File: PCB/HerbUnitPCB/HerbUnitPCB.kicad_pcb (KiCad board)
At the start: 2 copper layers, 43 parts, among them J1 USB_C_Receptacle_USB2.0_16P, J2 Barrel_Jack_Switch_Pin3Ring, J3 Conn_01x03_Pin, J4 SD_Card_Device, J5 Screw_Terminal_01x02, J6 Conn_01x03_Pin, SW1 SW_Push, SW2 SW_Push, SW3 SW_Push, U1 USBLC6-2P6, U2 ESP32-S3-WROOM-1, U3 AMS1117-5.0, U5 DHT11, U6 AP2112K-3.3

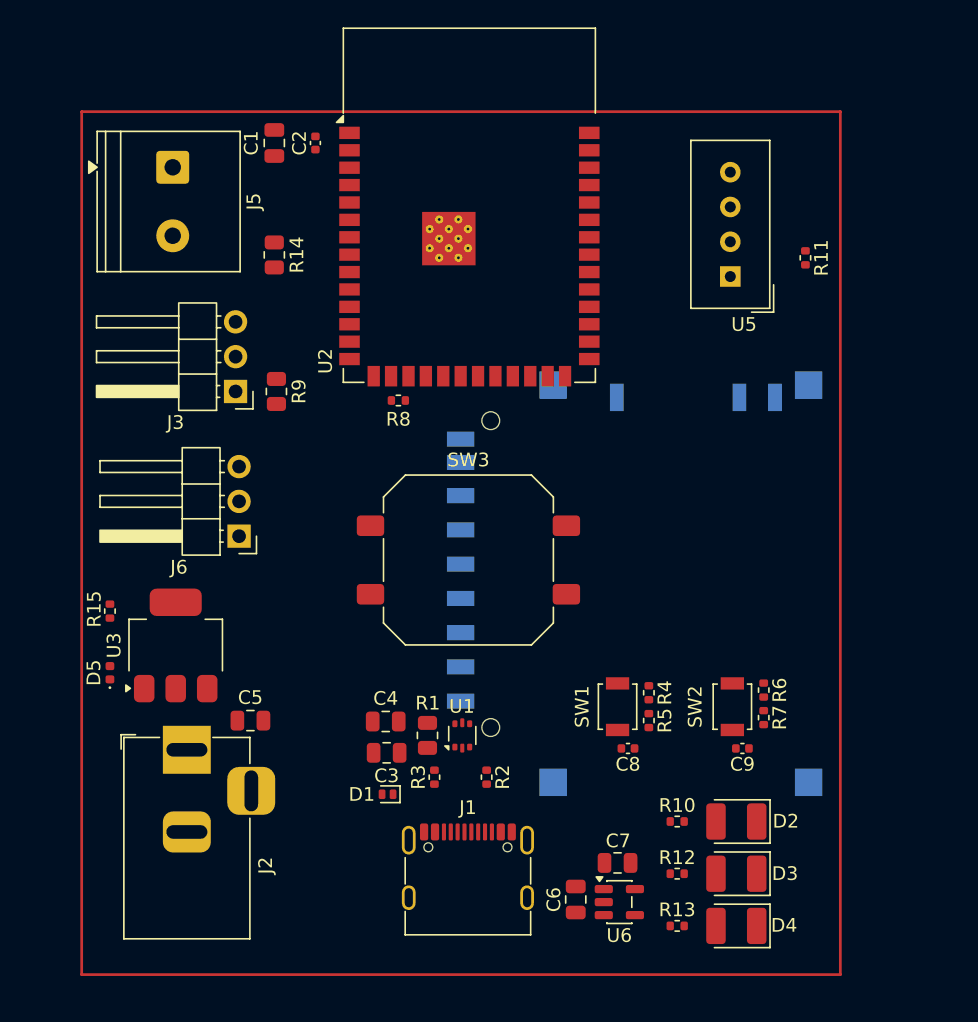
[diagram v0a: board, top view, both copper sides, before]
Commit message: PCB Routed + Silkscreen
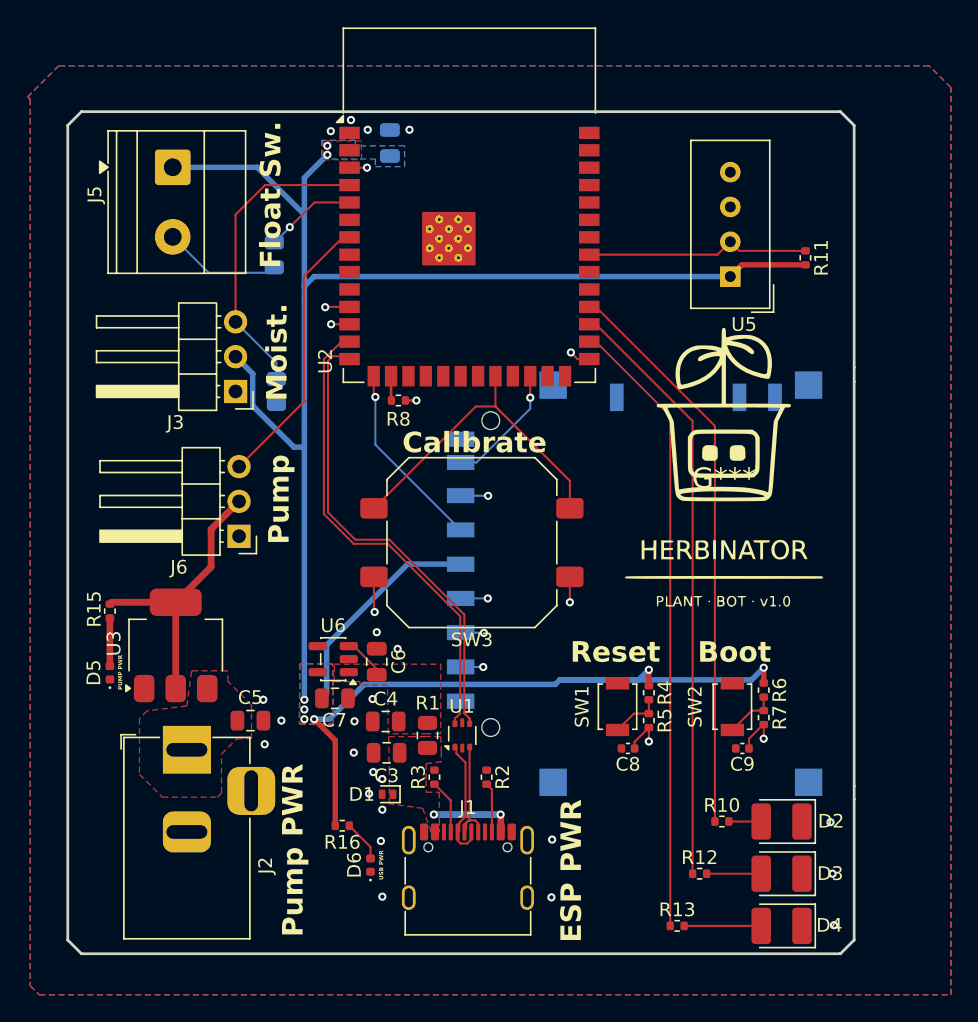
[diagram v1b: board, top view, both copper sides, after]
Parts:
- added D6: Green LED, LED_SMD:LED_0402_1005Metric, F.Cu at (160.0, 89.5)
- added G***: LOGO, LOGO, F.Cu at (185.8, 61.3)
- added G***: LOGO, LOGO, B.Cu at (167.2, 44.6)
- added G***: LOGO, LOGO, B.Cu at (184.0, 89.6)
- added R16: 2k, Resistor_SMD:R_0402_1005Metric, F.Cu at (158.0, 86.7)
- C1, C2, R14, R9: moved to B.Cu
- J5: footprint TerminalBlock_Philmore:TerminalBlock_Philmore_TB132_1x02_P5.00mm_Horizontal -> TerminalBlock_Phoenix:TerminalBlock_Phoenix_MKDS-1,5-2-5.08_1x02_P5.08mm_Horizontal
- moved U6 27.4 mm to (157.3, 74.5), turned to 180 degrees
- moved C7 23.9 mm to (157.4, 77.4), turned to 0 degrees
- moved C6 22.6 mm to (160.5, 74.7), turned to 90 degrees
- moved C1 8.44 mm to (161.4, 36.8)
- moved D2 3.30 mm to (190.0, 86.4)
- moved D3 3.30 mm to (190.0, 90.2)
- moved D4 3.30 mm to (190.0, 94.0)
- moved R10 3.26 mm to (185.7, 86.4)
- moved C2 2.55 mm to (158.5, 36.7)
- moved R12 1.64 mm to (184.0, 90.2)
- moved SW3 1.30 mm to (167.4, 66.0)
- turned C4 to 180 degrees
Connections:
- net Net-(D1-K) renamed VBUS
- net Net-(U3-VI) renamed JACK_BUS
- R10 pad 1: RedLED -> GreenLED
- R13 pad 1: GreenLED -> RedLED
- U2 pad 18: WaterRead -> unconnected-(U2-IO10-Pad18)
- U2 pad 19: RedLED -> unconnected-(U2-IO11-Pad19)
- U2 pad 20: BlueLED -> unconnected-(U2-IO12-Pad20)
- U2 pad 21: GreenLED -> unconnected-(U2-IO13-Pad21)
- U2 pad 22: unconnected-(U2-IO14-Pad22) -> CalibrationButton
- U2 pad 28: unconnected-(U2-IO35-Pad28) -> RedLED
- U2 pad 29: unconnected-(U2-IO36-Pad29) -> BlueLED
- U2 pad 30: unconnected-(U2-IO37-Pad30) -> GreenLED
- U2 pad 33: unconnected-(U2-IO40-Pad33) -> TempSensor
- U2 pad 5: TempSensor -> WaterRead
- U2 pad 6: CalibrationButton -> unconnected-(U2-IO6-Pad6)
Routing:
- net +3.3V_USB: track 0.00 -> 165.5 mm, vias 0 -> 8
- net En: track 0.00 -> 54.7 mm, vias 0 -> 2
- net RedLED: track 0.00 -> 45.4 mm
- net BlueLED: track 0.00 -> 43.5 mm
- net GreenLED: track 0.00 -> 41.6 mm
- net BootMode1: track 0.00 -> 38.8 mm, vias 0 -> 2
- net SD_CS: track 0.00 -> 34.9 mm, vias 0 -> 2
- net USB_D-: track 0.00 -> 34.7 mm
- net USB_D+: track 0.00 -> 34.0 mm
- net SD_MOSI: track 0.00 -> 30.2 mm, vias 0 -> 2
- net CalibrationButton: track 0.00 -> 23.8 mm
- net MoistureRead: track 0.00 -> 22.4 mm
- net +5V_JACK: track 0.00 -> 20.4 mm
- net PumpMotor: track 0.00 -> 20.4 mm
- net TempSensor: track 0.00 -> 16.4 mm
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- added copper zone on B.Cu, net +3.3V_USB
- added copper zone on F.Cu, net +3.3V_USB
- added copper zone on F.Cu, net +5V
- added copper zone on B.Cu, net GND
- added copper zone on F.Cu, net GND
- added copper zone on In1.Cu, net GND
- added copper zone on In2.Cu, net GND
- added copper zone on F.Cu, net JACK_BUS
- added copper zone on F.Cu, net VBUS
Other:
- board outline added: 57.4 x 61.5 mm
- copper layers 2 -> 4
- board text added: "Boot"
- board text added: "Calibrate"
- board text added: "ESP PWR"
- board text added: "Float Sw."
- board text added: "Moist."
- board text added: "PUMP PWR"
- board text added: "Pump"
- board text added: "Pump PWR"
- board text added: "Reset"
- board text added: "SD Card Reader"
- board text added: "USB PWR"
